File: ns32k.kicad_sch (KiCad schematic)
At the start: 44 parts, among them U1 NS32201, U10 74AHC373, U11 74AHC373, U12 74AHC138, U13 AS6C6416-55, U15 MX29LV040C, U16 MX29LV040C, U19 74AHC138, U20 74AHC1G08, U3 NS32016, U4 NS32082, U5 NS32202, U6 74AHC08, U7 74AHC245, U8 74AHC245, U9 74AHC373

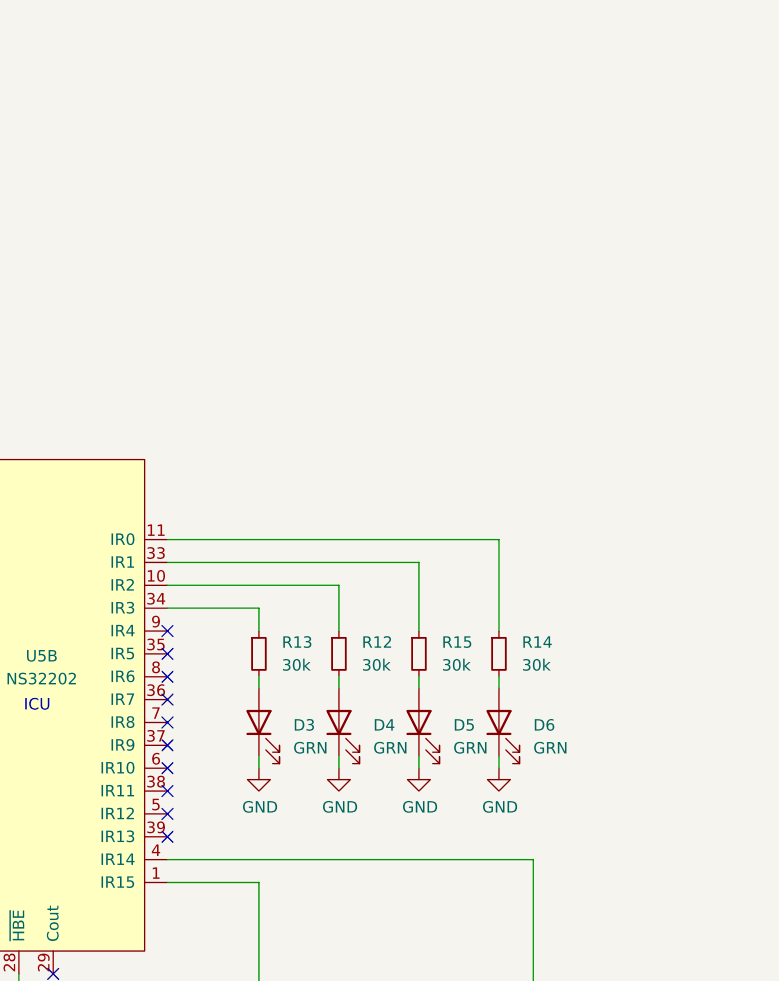
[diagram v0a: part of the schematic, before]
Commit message: cleanups, DRC
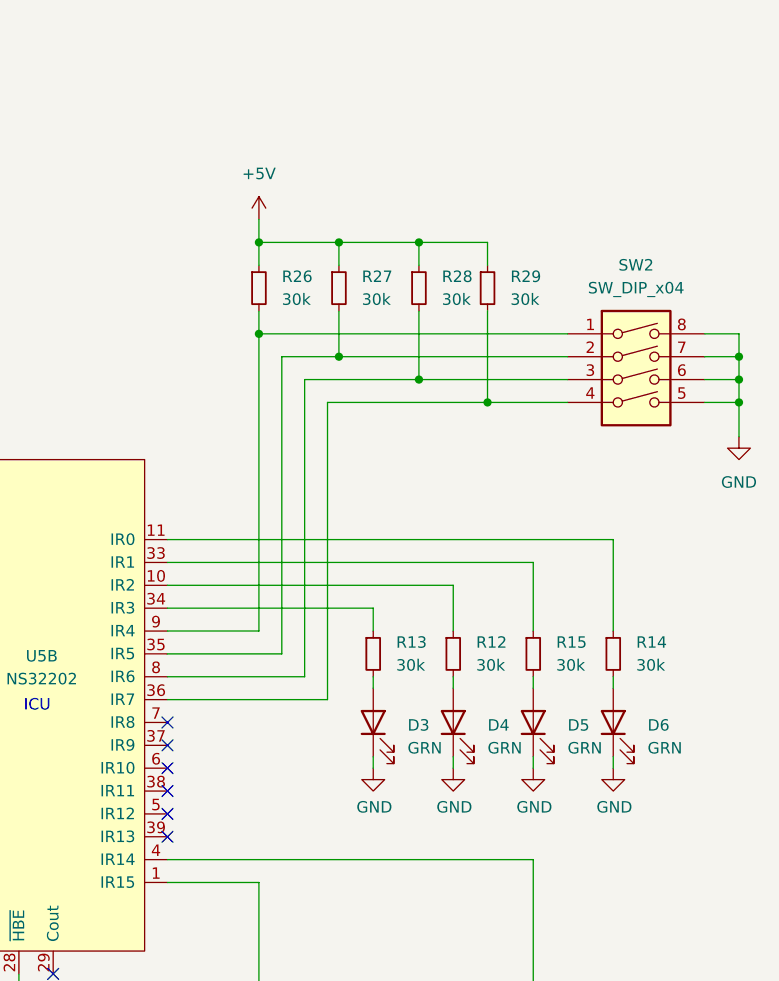
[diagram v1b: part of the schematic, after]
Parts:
- added R26, R27, R28, R29: 30k, Resistor_SMD:R_0402_1005Metric, symbol Device:R_Small
- added SW2: SW_DIP_x04, Button_Switch_SMD:SW_DIP_SPSTx04_Slide_Copal_CHS-04B_W7.62mm_P1.27mm, symbol Switch:SW_DIP_x04
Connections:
- net +5V: now also R26.1, R27.1, R28.1, R29.1
- net GND: now also SW2.5, SW2.6, SW2.7, SW2.8
- net at U5.35 (IR5): now also R27.2, SW2.2
- net at U5.36 (IR7): now also R29.2, SW2.4
- net at U5.8 (IR6): now also R28.2, SW2.3
- net at U5.9 (IR4): now also R26.2, SW2.1
- no-connect marks 25 -> 21
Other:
- moved on the sheet: D3, D4, D5, D6, R12, R13, R14, R15
